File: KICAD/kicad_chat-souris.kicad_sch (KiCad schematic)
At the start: 0 parts

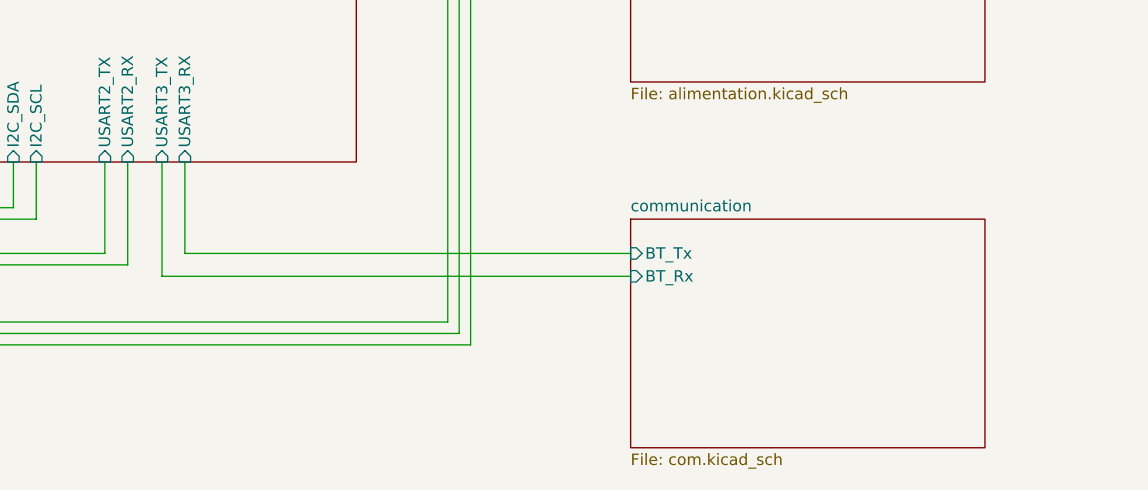
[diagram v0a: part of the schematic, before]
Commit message: PCB finalized
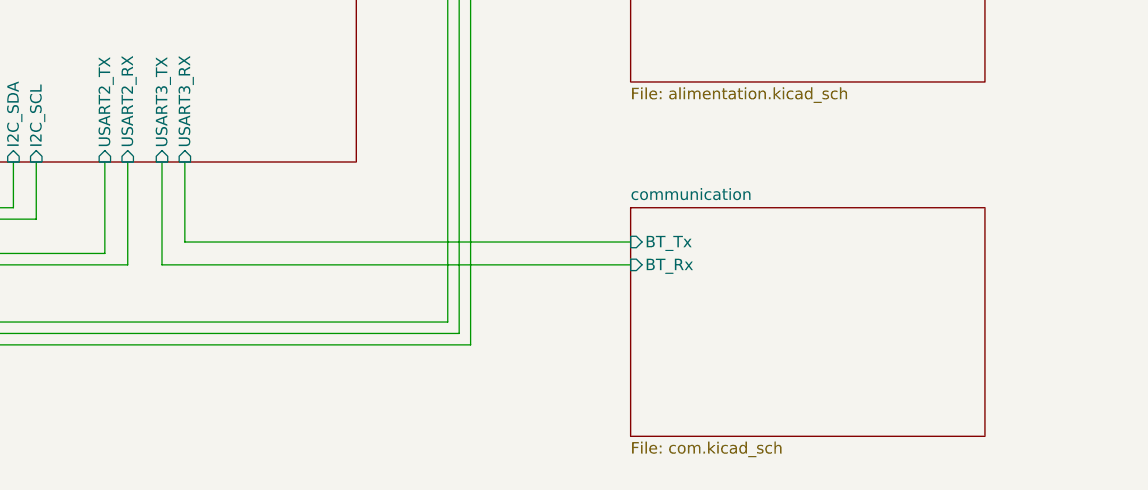
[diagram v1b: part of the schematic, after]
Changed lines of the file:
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@@
     (stroke (width 0) (type default))
   )
-  (wire (pts (xy 161.29 111.76) (xy 210.82 111.76))
-    (stroke (width 0) (type default))
-  )
-  (wire (pts (xy 161.29 101.6) (xy 161.29 111.76))
+  (wire (pts (xy 161.29 110.49) (xy 210.82 110.49))
+    (stroke (width 0) (type default))
+  )
+  (wire (pts (xy 161.29 101.6) (xy 161.29 110.49))
     (stroke (width 0) (type default))
   )
@@
     (stroke (width 0) (type default))
   )
-  (wire (pts (xy 210.82 114.3) (xy 158.75 114.3))
+  (wire (pts (xy 210.82 113.03) (xy 158.75 113.03))
     (stroke (width 0) (type default))
   )
@@
     (stroke (width 0) (type default))
   )
-  (wire (pts (xy 158.75 101.6) (xy 158.75 114.3))
+  (wire (pts (xy 158.75 101.6) (xy 158.75 113.03))
     (stroke (width 0) (type default))
   )
@@
     )
   )
-  (sheet (at 210.82 107.95) (size 39.37 25.4) (fields_autoplaced)
+  (sheet (at 210.82 106.68) (size 39.37 25.4) (fields_autoplaced)
     (stroke (width 0.1524) (type solid))
     (fill (color 0 0 0 0.0000))
-    (property "Sheetname" "communication" (at 210.82 107.2384 0)
+    (property "Sheetname" "communication" (at 210.82 105.9684 0)
       (effects (font (size 1.27 1.27)) (justify left bottom))
     )
-    (property "Sheetfile" "com.kicad_sch" (at 210.82 133.9346 0)
+    (property "Sheetfile" "com.kicad_sch" (at 210.82 132.6646 0)
       (effects (font (size 1.27 1.27)) (justify left top))
     )
-    (pin "BT_Tx" input (at 210.82 111.76 180)
-      (effects (font (size 1.27 1.27)) (justify left))
-    )
-    (pin "BT_Rx" input (at 210.82 114.3 180)
-      (effects (font (size 1.27 1.27)) (justify left))
-    )
+    (pin "BT_Tx" input (at 210.82 110.49 180)
+      (effects (font (size 1.27 1.27)) (justify left))
+    )
+    (pin "BT_Rx" input (at 210.82 113.03 180)
+      (effects (font (size 1.27 1.27)) (justify left))
+    )
